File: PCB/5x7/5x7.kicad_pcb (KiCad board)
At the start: 2 copper layers, 14.5 x 14.5 mm, 51 parts, among them J1 Conn_01x03, J2 Conn_01x03

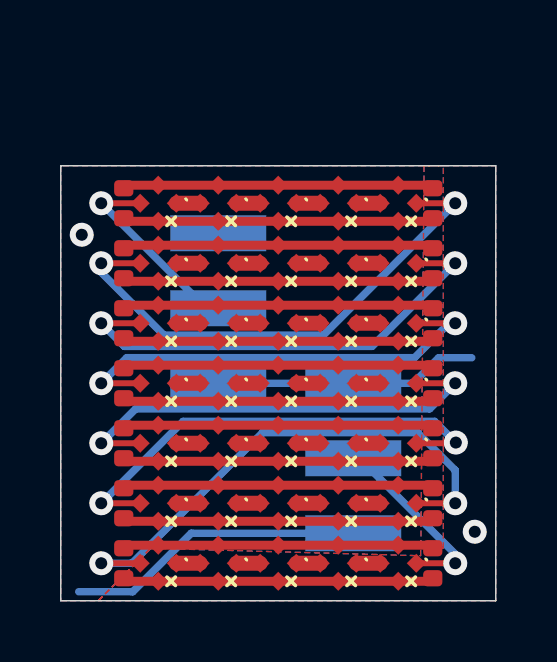
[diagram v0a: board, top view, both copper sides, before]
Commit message: New layout
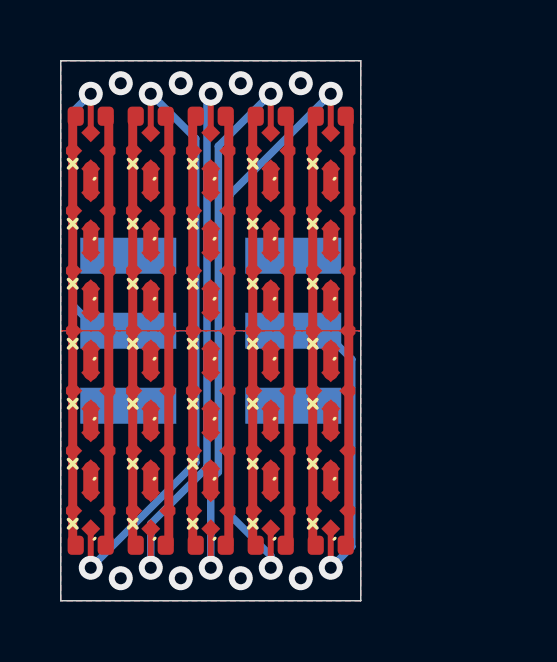
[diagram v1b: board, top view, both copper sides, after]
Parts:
- removed C11, C12, C13, C14: 330nF, RevK:C_0402
- moved C2 16.1 mm to (101.0, 98.2), turned to 0 degrees
- moved C4 13.3 mm to (103.0, 98.2), turned to 0 degrees
- moved C9 12.9 mm to (109.0, 83.8), turned to 0 degrees
- moved D5 12.0 mm to (101.0, 93.0), turned to 135 degrees
- moved D29 11.8 mm to (109.0, 85.0), turned to 135 degrees
- moved D31 11.3 mm to (109.0, 89.0), turned to 135 degrees
- moved C6 10.5 mm to (105.0, 98.2), turned to 0 degrees
- moved C7 10.2 mm to (107.0, 83.8), turned to 0 degrees
- moved D30 10.0 mm to (109.0, 87.0), turned to 135 degrees
- moved D22 9.91 mm to (107.0, 85.0), turned to 135 degrees
- moved D4 9.28 mm to (101.0, 91.0), turned to 135 degrees
- moved D7 9.28 mm to (101.0, 97.0), turned to 135 degrees
- moved D14 8.84 mm to (103.0, 97.0), turned to 135 degrees
- moved D32 8.61 mm to (109.0, 91.0), turned to 135 degrees
- moved D15 8.49 mm to (105.0, 85.0), turned to 135 degrees
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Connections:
- net VDD renamed VCC
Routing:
- net Net-(D7-O): track 0.80 -> 20.5 mm, vias 0 -> 2
- net Net-(D28-O): track 0.80 -> 20.4 mm, vias 0 -> 2
- net Net-(D21-O): track 0.80 -> 19.2 mm, vias 0 -> 2
- net Net-(D14-O): track 0.80 -> 19.2 mm, vias 0 -> 2
- net Net-(D30-O): track 17.8 -> 0.80 mm, vias 2 -> 0
- net Net-(D5-O): track 17.4 -> 0.80 mm, vias 2 -> 0
- net Net-(D25-O): track 15.9 -> 0.80 mm, vias 2 -> 0
- net Net-(D10-O): track 15.9 -> 0.80 mm, vias 2 -> 0
- net Net-(D15-O): track 15.2 -> 0.80 mm, vias 2 -> 0
- net Net-(D20-O): track 15.2 -> 0.80 mm, vias 2 -> 0
- net GND: track 82.1 -> 71.5 mm, vias 1 -> 4
- net VCC: track 80.9 -> 71.5 mm, vias 1 -> 4
- net Net-(D35-O): track 6.33 -> 10.9 mm
- net Net-(D1-I): track 6.65 -> 10.8 mm
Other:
- board size 14.5 x 14.5 mm -> 10 x 18 mm
